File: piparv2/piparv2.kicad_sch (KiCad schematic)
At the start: 40 parts, among them SW1 SW_Wuerth_450301014042, U1 Seeeduino Xiao nRF52840

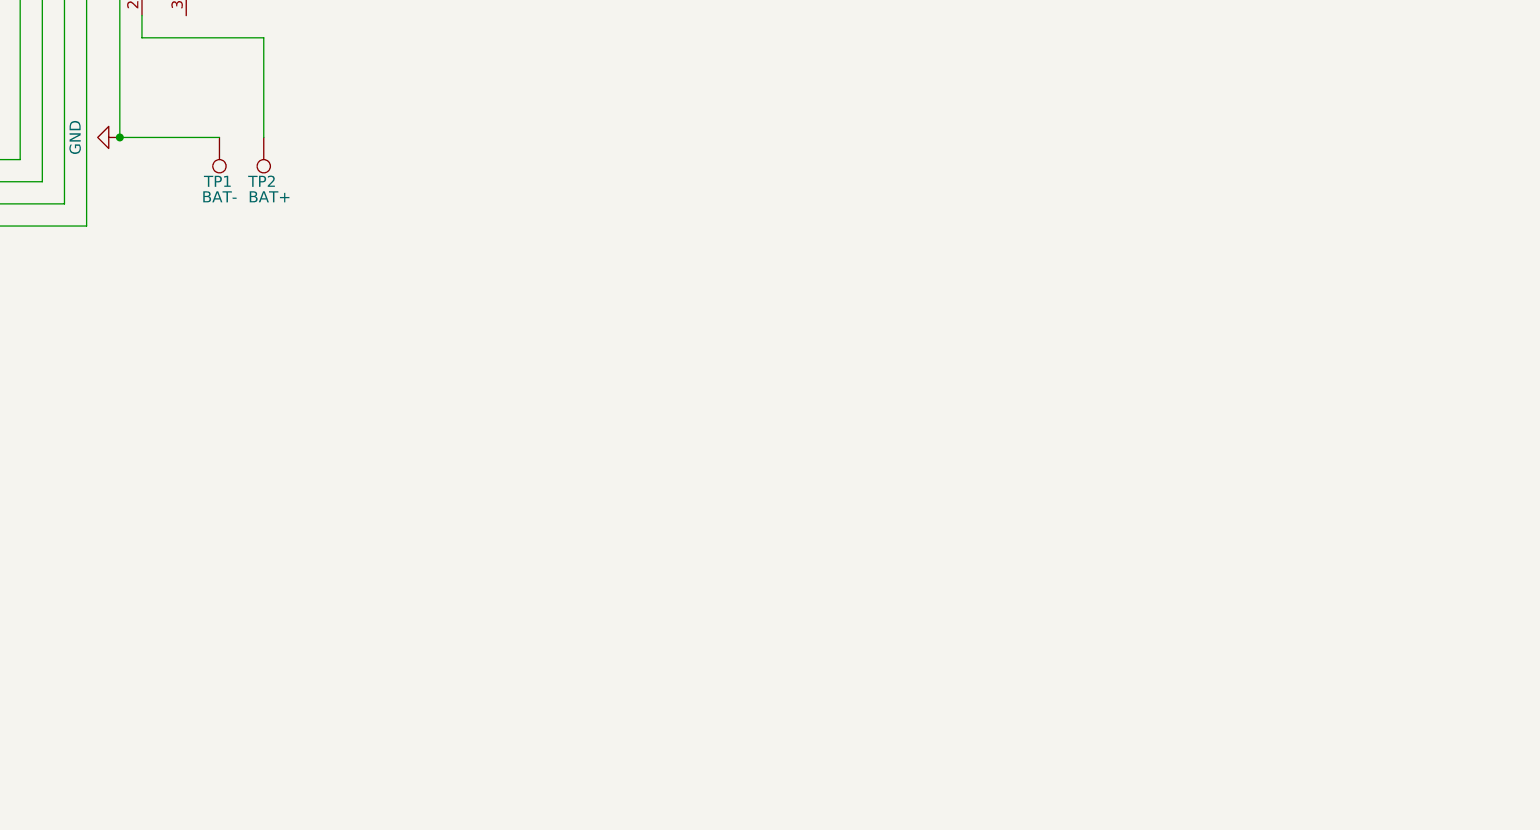
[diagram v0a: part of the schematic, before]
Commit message: adds macropad
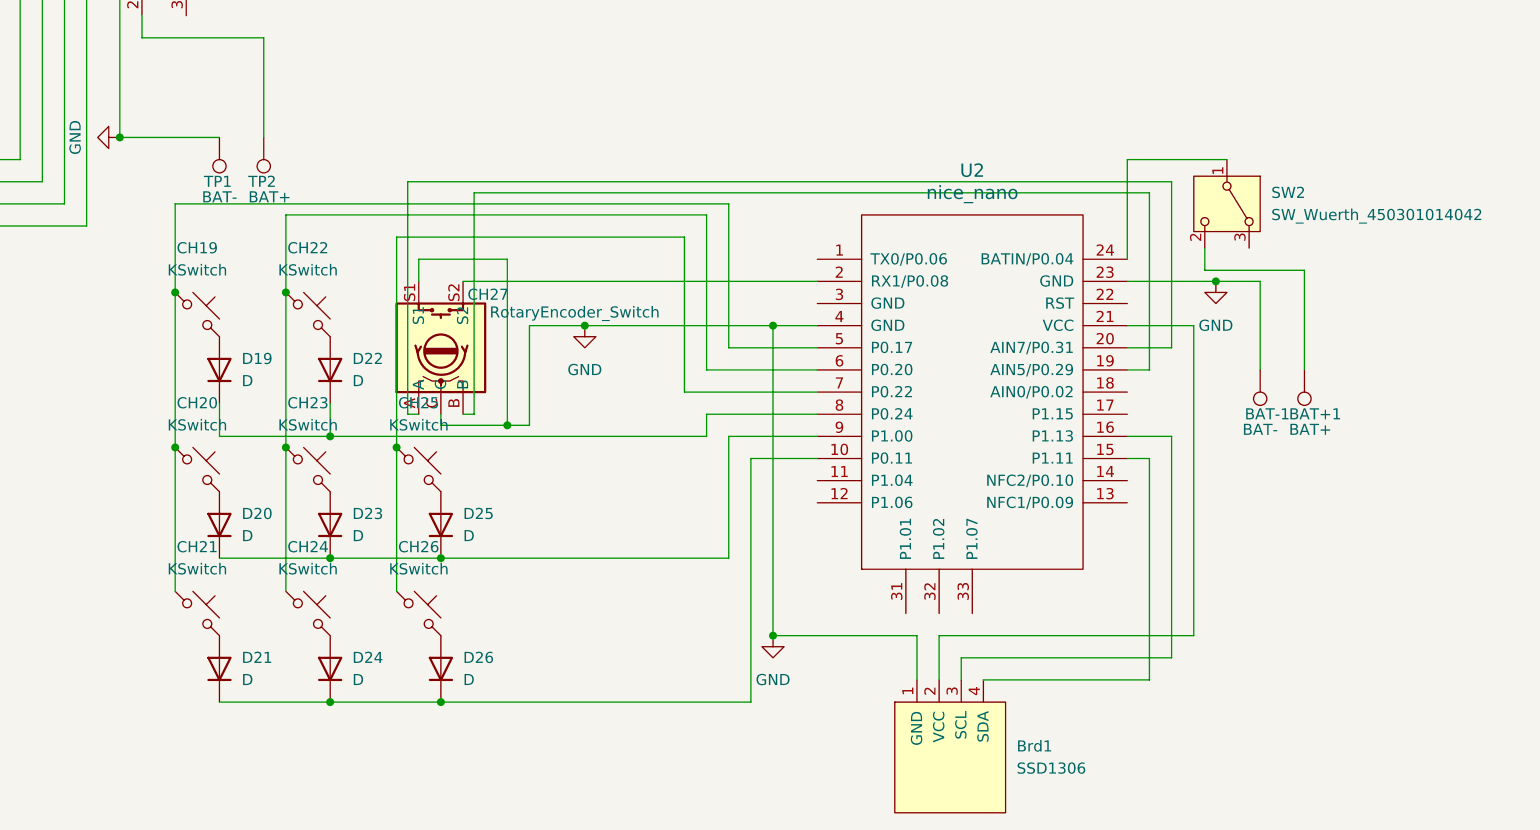
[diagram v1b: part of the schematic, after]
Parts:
- added BAT+1: BAT+, TestPoint:TestPoint_THTPad_D2.0mm_Drill1.0mm, symbol Connector:TestPoint
- added BAT-1: BAT-, TestPoint:TestPoint_THTPad_2.0x2.0mm_Drill1.0mm, symbol Connector:TestPoint
- added Brd1: SSD1306, SSD1306:128x64OLED_0.91, symbol SSD1306-128x64_OLED:SSD1306
- added CH19, CH20, CH21, CH22, CH23, CH24, CH25, CH26: KSwitch, keyswitches:Kailh_socket_PG1350_reversible, symbol marbastlib-choc:choc_v1_SW_HS_CPG135001S30
- added CH27: RotaryEncoder_Switch, Rotary_Encoder:RotaryEncoder_Bourns_Vertical_PEL11L-4xxxF-Sxxxx_1, symbol Device:RotaryEncoder_Switch
- added D19, D20, D21, D22, D23, D24, D25, D26: D, Diode_SMD:Nexperia_CFP3_SOD-123W, symbol Device:D
- added SW2: SW_Wuerth_450301014042, Button_Switch_SMD:SW_SPDT_PCM12, symbol Switch:SW_Wuerth_450301014042
- added U2: nice_nano, nice-nano-kicad:nice_nano, symbol nice_nano:nice_nano
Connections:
- net GND: now also BAT-1.1, Brd1.1 (GND), CH27.C, CH27.S1, U2.23 (GND), U2.4 (GND)
- new net: CH22.1, CH23.1, CH24.1, U2.6 (P0.20)
- new net: CH22.2, D22.2 (A)
- new net: BAT+1.1, SW2.2 (C)
- new net: Brd1.2 (VCC), U2.21 (VCC)
- new net: Brd1.3 (SCL), U2.16 (P1.13)
- new net: Brd1.4 (SDA), U2.15 (P1.11)
- new net: D19.1 (K), D22.1 (K), U2.8 (P0.24)
- new net: CH24.2, D24.2 (A)
- new net: D21.1 (K), D24.1 (K), D26.1 (K), U2.10 (P0.11)
- new net: CH26.2, D26.2 (A)
- new net: CH27.B, U2.19 (AIN5/P0.29)
- new net: CH27.S2, U2.2 (RX1/P0.08)
- new net: CH27.A, U2.20 (AIN7/P0.31)
- new net: SW2.1 (B), U2.24 (BATIN/P0.04)
- new net: CH19.1, CH20.1, CH21.1, U2.5 (P0.17)
- new net: CH25.1, CH26.1, U2.7 (P0.22)
- new net: D20.1 (K), D23.1 (K), D25.1 (K), U2.9 (P1.00)
- new net: CH19.2, D19.2 (A)
- new net: CH20.2, D20.2 (A)
- new net: CH25.2, D25.2 (A)
- new net: CH23.2, D23.2 (A)
- new net: CH21.2, D21.2 (A)

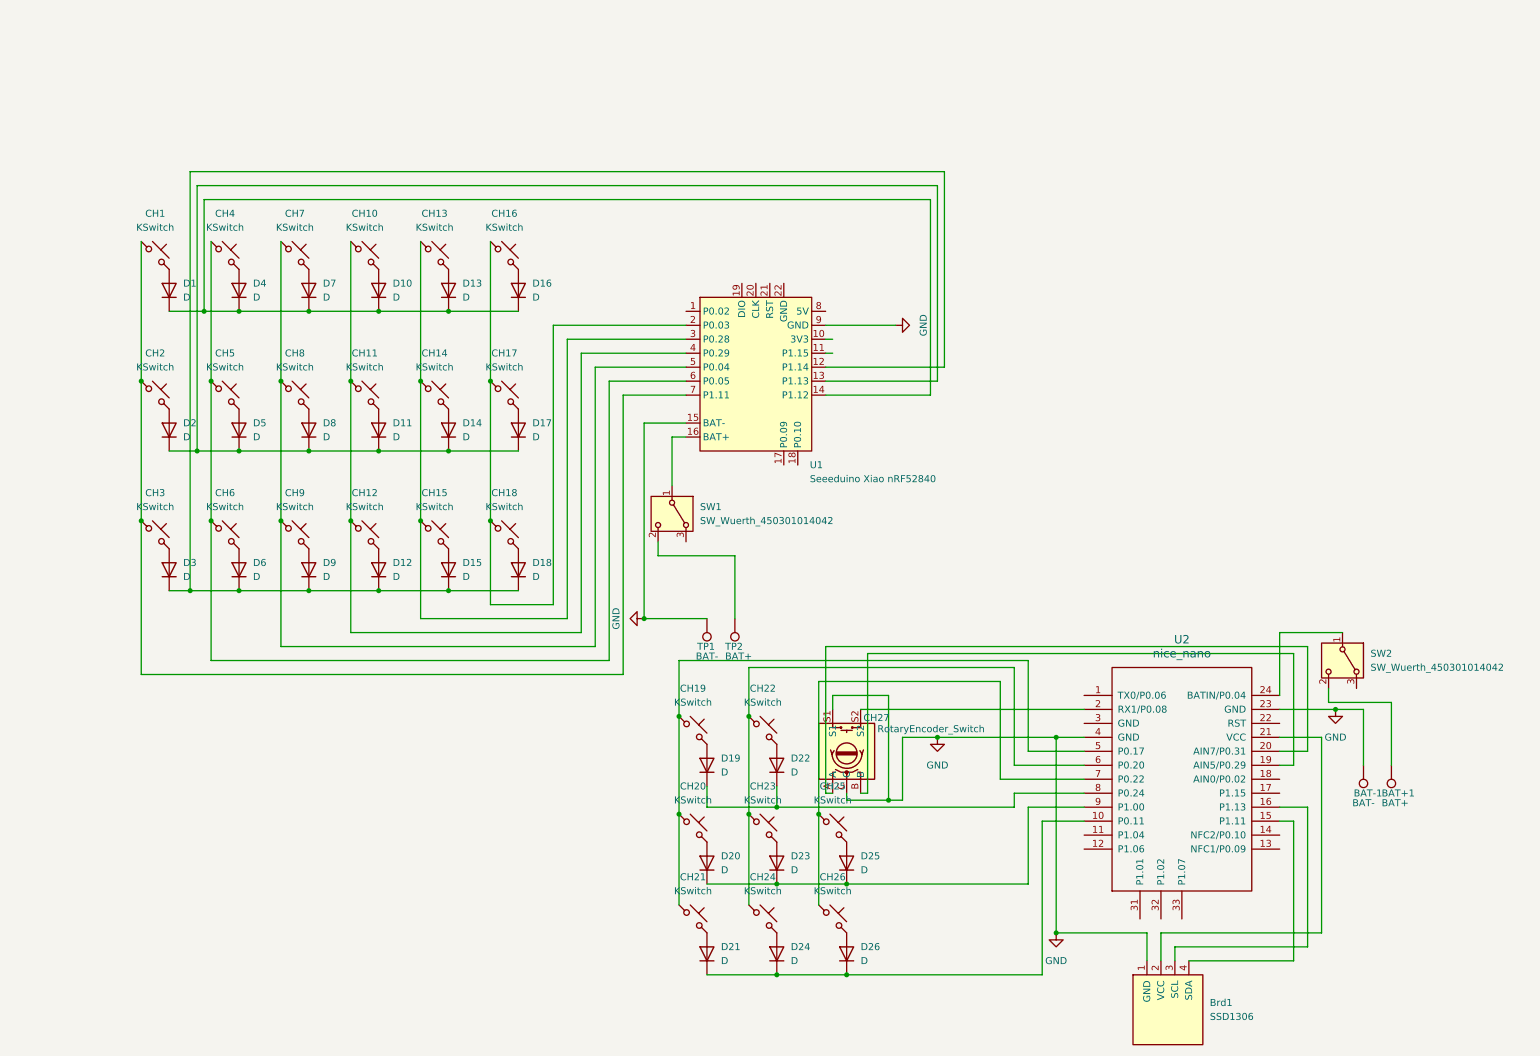
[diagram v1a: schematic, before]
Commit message: Improves handling of the kicad
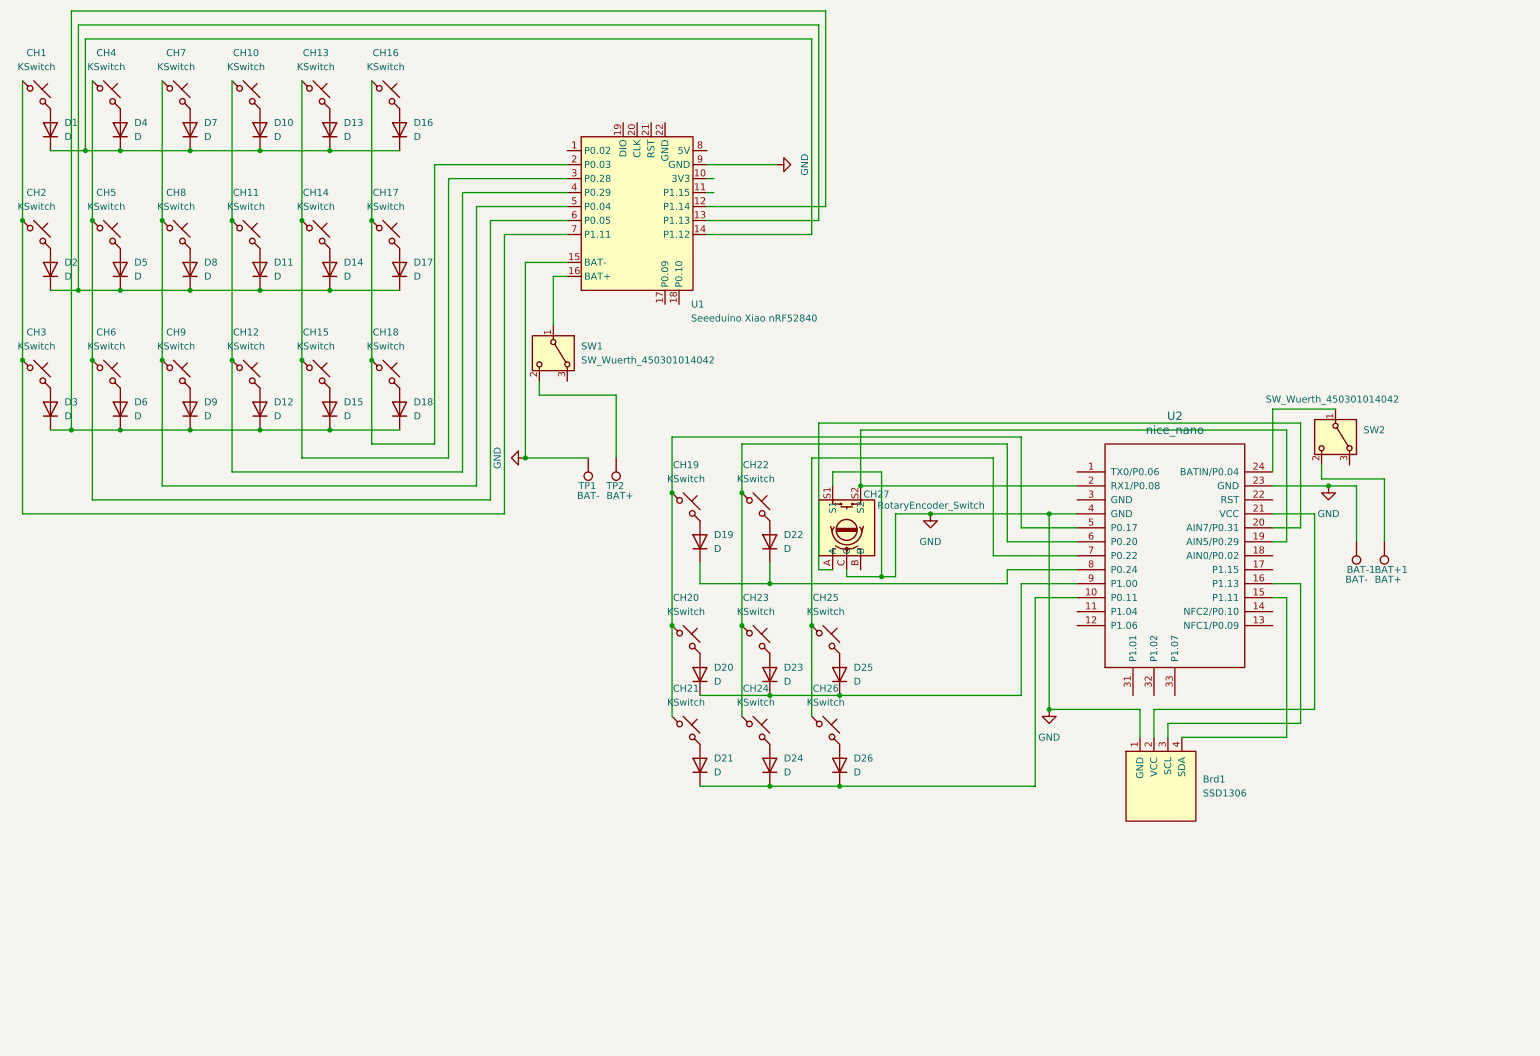
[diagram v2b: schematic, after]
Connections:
- net at U2.19 (AIN5/P0.29): now also CH27.S2, U2.2 (RX1/P0.08); no longer CH27.B
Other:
- moved on the sheet: BAT+1, BAT-1, Brd1, CH1, CH10, CH11, CH12, CH13, CH14, CH15, CH16, CH17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
